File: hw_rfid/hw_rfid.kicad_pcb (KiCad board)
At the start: 2 copper layers, 71.8 x 53.9 mm, 50 parts, among them IC1 XC9288A33CER-G, IC2 TPS610333DRLR, J1 Conn_01x02, J2 Conn_01x05, J3 Conn_01x04, J4 Conn_01x03, J5 Conn_01x08, Q1 2N7002, SW1 SW_Push, SW2 SW_Push, SW3 SW_Push, U1 STM32U031K6Ux, U2 AT45DB021E-SHN-T

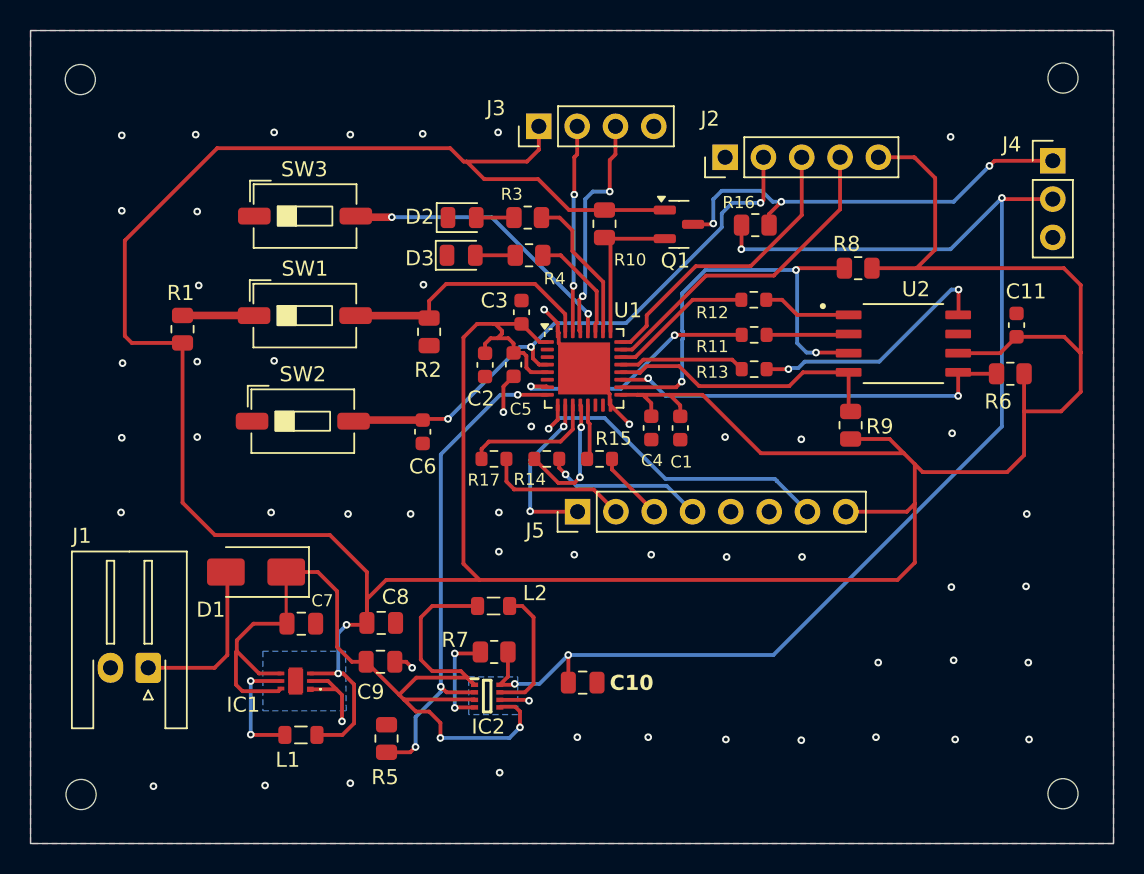
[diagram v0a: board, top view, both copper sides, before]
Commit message: vista pelo marcelo mas nao reorganizada
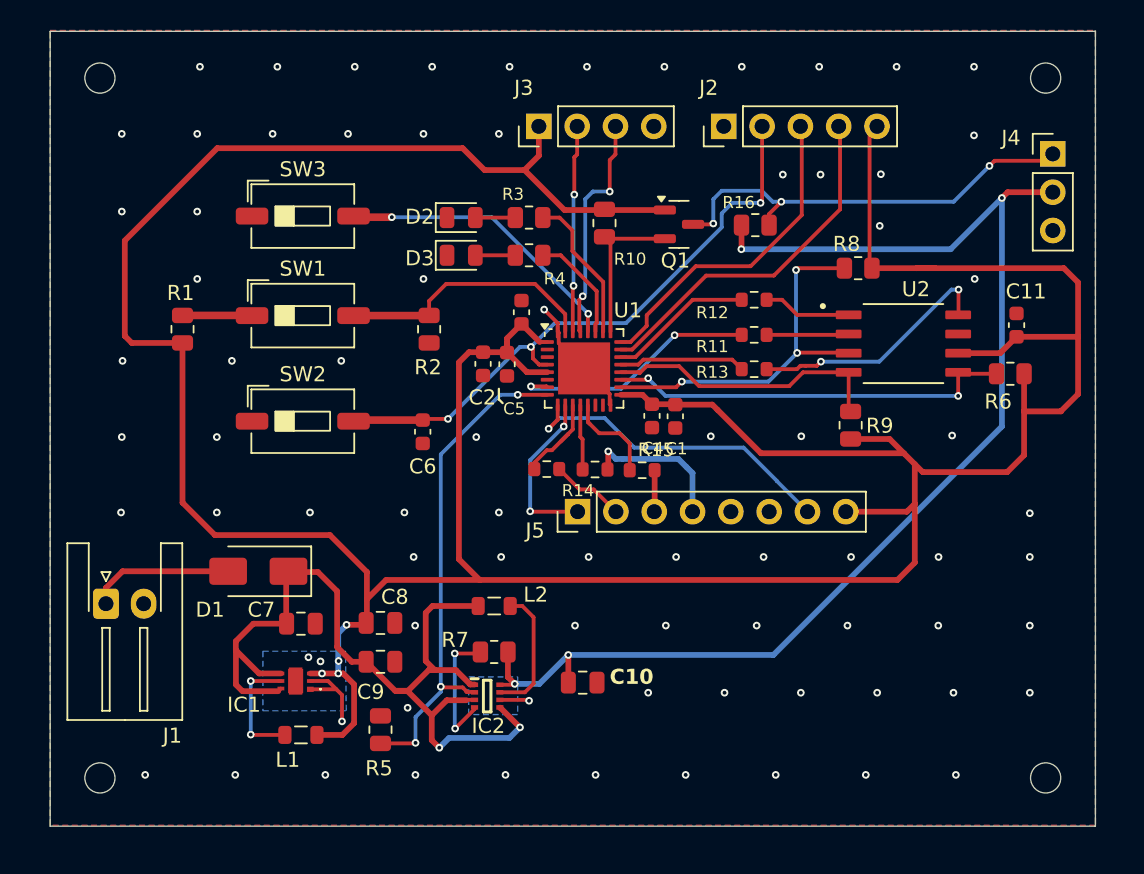
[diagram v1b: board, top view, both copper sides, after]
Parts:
- moved J1 5.09 mm to (79.0, 111.1), turned to 0 degrees
- moved R17 3.56 mm to (108.2, 102.2)
- moved R14 3.28 mm to (111.4, 102.2)
- moved R15 2.92 mm to (114.5, 102.2)
- moved J2 2.05 mm to (119.9, 79.5)
- moved REF** 1.67 mm to (78.5, 122.7)
- moved REF** 1.56 mm to (141.2, 122.7)
- moved REF** 1.30 mm to (78.5, 76.2)
- moved REF** 1.15 mm to (141.2, 76.2)
- moved C1 0.84 mm to (116.7, 98.7)
- moved C4 0.80 mm to (115.2, 98.7)
- moved R5 0.71 mm to (97.2, 119.5)
- moved J4 0.46 mm to (141.7, 81.3)
- moved C5 0.44 mm to (105.5, 95.2)
- moved R2 0.17 mm to (100.4, 92.9)
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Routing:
- net +3.3V: track 267.6 -> 256.1 mm, vias 2 -> 6
- net GND: track 22.4 -> 16.6 mm, vias 53 -> 77
- net /nRESET_FLASH: track 30.1 -> 24.9 mm
- net Net-(J5-Pin_2): track 9.60 -> 4.93 mm
- net /SPI1_MISO_RFID: track 8.73 -> 4.32 mm, vias 2 -> 0
- net +BATT: track 64.1 -> 60.1 mm
- net /SPI1_MOSI_RFID: track 3.68 -> 6.42 mm
- net /SPI1_SCK_RFID: track 8.86 -> 6.21 mm
- net /SWDIO: track 21.8 -> 23.9 mm
- net /SWCLK: track 19.7 -> 21.8 mm
- net /NRST: track 38.6 -> 40.6 mm
- net Net-(IC2-PG): track 6.81 -> 8.71 mm
- net Net-(J5-Pin_3): track 4.66 -> 2.76 mm
- net Net-(D1-A): track 11.1 -> 9.61 mm
- net Net-(J5-Pin_4): track 10.7 -> 9.97 mm
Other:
- board size 71.8 x 53.9 mm -> 69.3 x 52.7 mm
